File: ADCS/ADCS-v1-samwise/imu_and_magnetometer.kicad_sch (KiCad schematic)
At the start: 3 parts, among them U10 RM3100CB, U11 BMI270

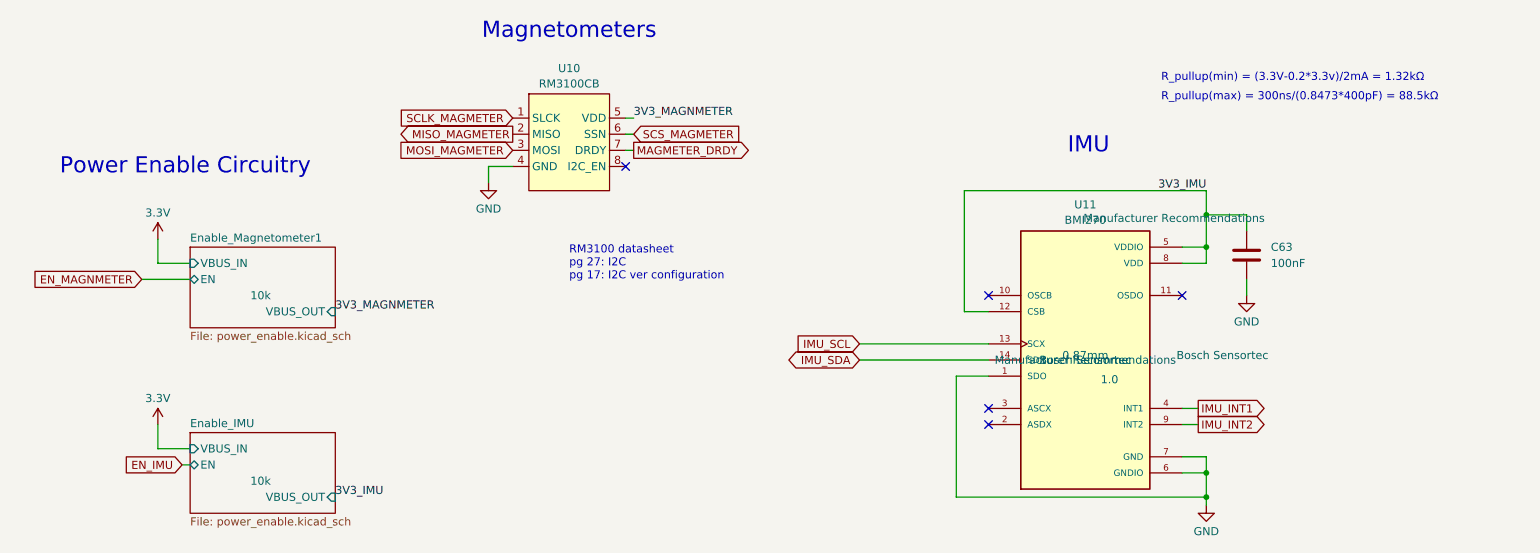
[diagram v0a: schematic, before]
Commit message: ver 1.5
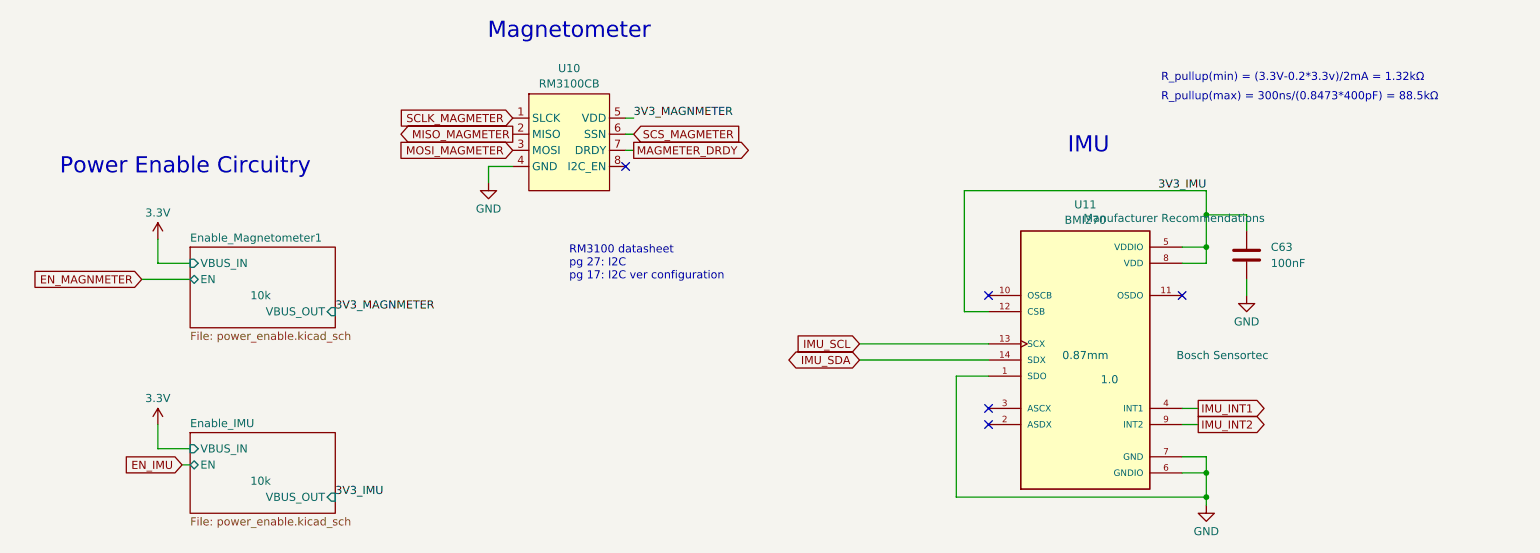
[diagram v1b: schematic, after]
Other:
- note added: "Magnetometer"
- note removed: "Magnetometers"
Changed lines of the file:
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@@
 		(title "ADCS Main Board")
 		(date "2025-05-21")
-		(rev "1.4")
+		(rev "1.5")
 		(company "Stanford Student Space Initiative")
 		(comment 1 "Sage Wu")
@@
 		)
 	)
-	(text "Magnetometers"
+	(text "Magnetometer"
 		(exclude_from_sim no)
 		(at 113.03 65.024 0)
@@
 					(size 1.27 1.27)
 				)
+				(hide yes)
 			)
 		)
@@
 					(size 1.27 1.27)
 				)
-			)
-		)
+				(hide yes)
+			)
+		)
